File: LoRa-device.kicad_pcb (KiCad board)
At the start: 2 copper layers, 86.4 x 50.8 mm, 90 parts, among them J1 USB_C_Receptacle_USB2.0_14P, J2 Conn_01x02_Pin, J3 Conn_01x12_Pin, J4 Conn_01x14_Pin, J6 Conn_01x04_Pin, Q1 AO3401A, Q2 S8050, U1 ESP32-S3, U2 W25Q128JVS, U3 MCP73831-2-OT, U4 AMS1117-3.3, U5 Ai-Thinker-Ra-01, U6 BME280, U7 L70-R, Y1 32.768 kHz, Y2 40MHz(10ppm)

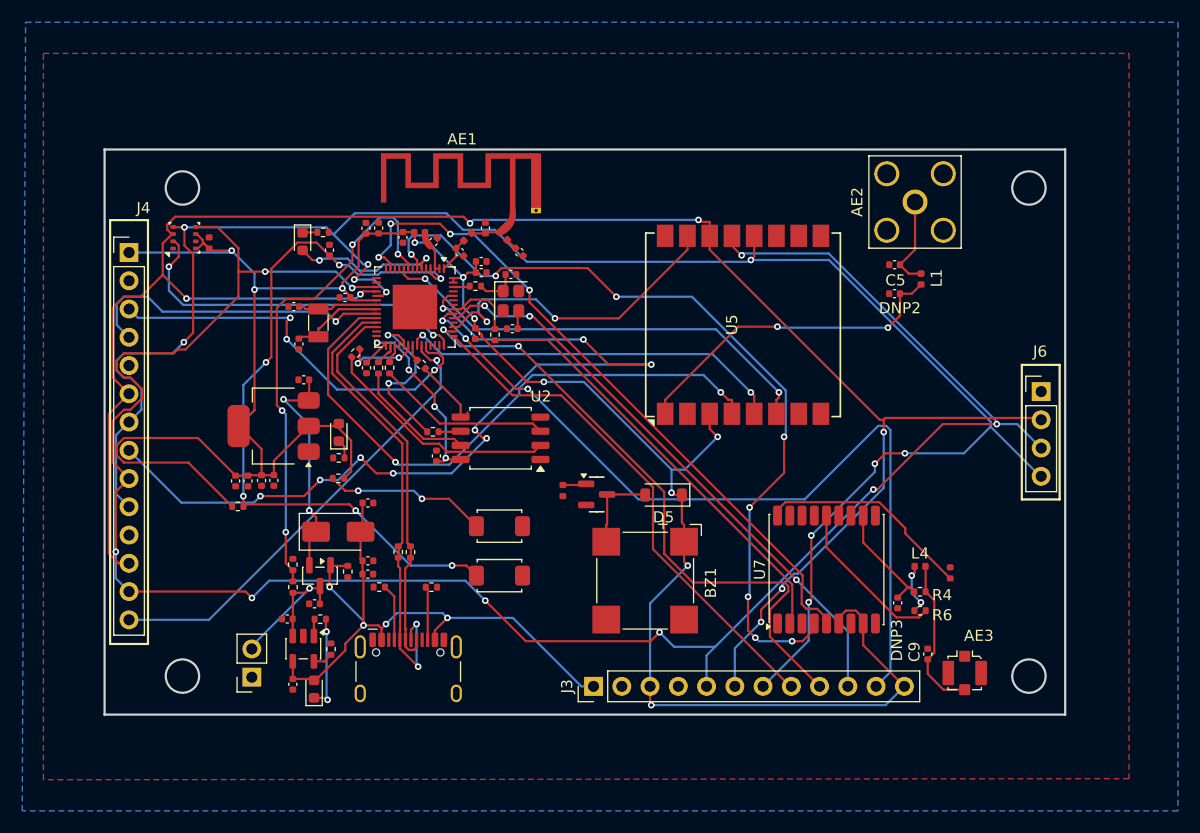
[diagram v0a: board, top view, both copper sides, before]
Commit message: First routing
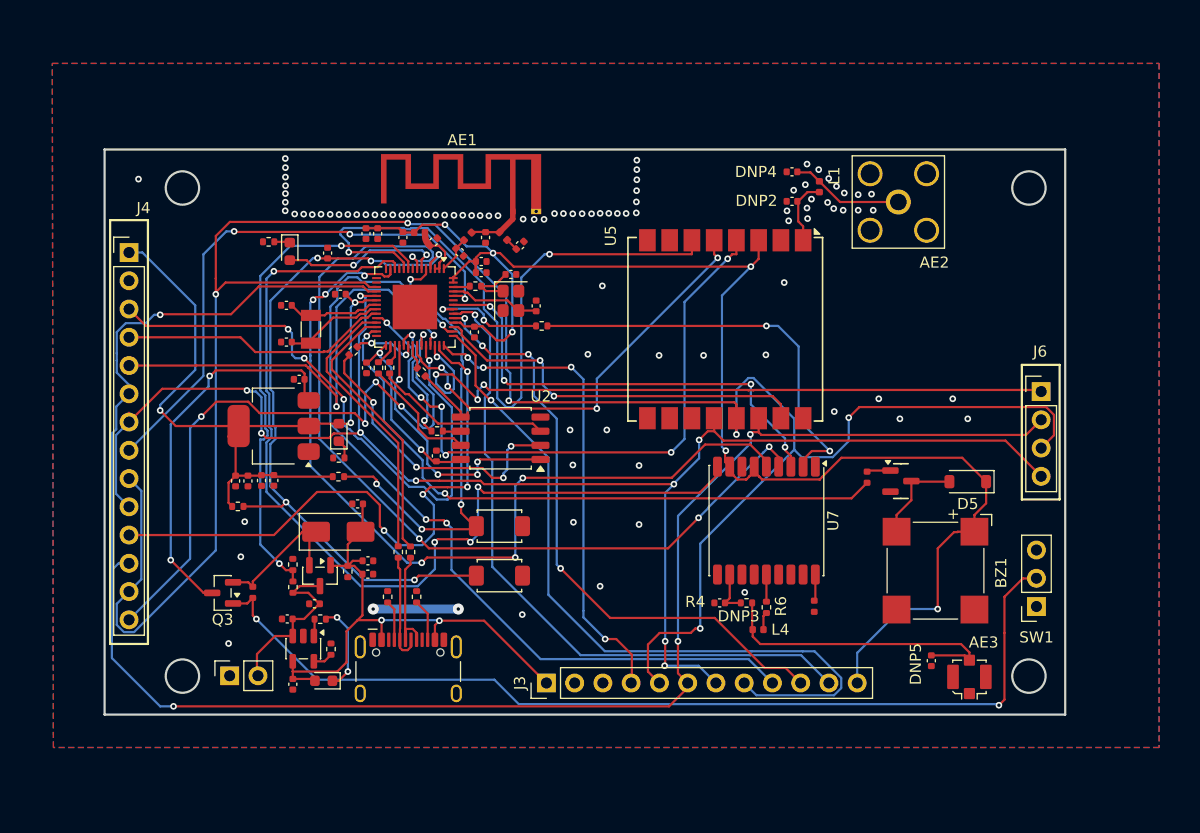
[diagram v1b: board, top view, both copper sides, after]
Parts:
- removed C1: 100nF, PCM_JLCPCB:C_0402
- removed C5, C9: 15pF, Capacitor_SMD:C_0402_1005Metric
- removed U6: BME280, PCM_JLCPCB:Bosch_LGA-8_2.5x2.5mm_P0.65mm_ClockwisePinNumbering
- added DNP4: ~, Capacitor_SMD:C_0402_1005Metric, F.Cu at (163.7, 75.8)
- added DNP5: ~, Capacitor_SMD:C_0402_1005Metric, F.Cu at (176.2, 119.8)
- added Q3: AO3401A, Package_TO_SOT_SMD:SOT-23, F.Cu at (112.5, 113.7)
- added R7: 100kΩ, PCM_JLCPCB:R_0402, F.Cu at (115.2, 113.7)
- added SW1: SW_Nidec_CAS-120A1, Connector_PinSocket_2.54mm:PinSocket_1x03_P2.54mm_Vertical, F.Cu at (185.7, 114.9)
- DNP2, DNP3: value 15pF -> ~
- moved Q2 27.4 mm to (173.5, 103.7)
- moved D5 27.4 mm to (179.5, 103.7)
- moved R5 27.4 mm to (170.4, 103.3)
- moved BZ1 26.1 mm to (176.6, 111.7)
- moved DNP3 16.0 mm to (157.2, 114.6), turned to 180 degrees
- moved L4 15.6 mm to (160.7, 117.0), turned to 180 degrees
- moved R4 15.6 mm to (159.6, 114.6)
- moved R6 13.8 mm to (161.4, 115.0), turned to 90 degrees
- moved R3 12.6 mm to (165.7, 114.9), turned to -90 degrees
- moved DNP2 12.4 mm to (163.7, 78.5)
- moved L1 12.3 mm to (166.2, 77.2)
- moved U7 6.97 mm to (161.4, 107.2), turned to -90 degrees
- moved R25 4.97 mm to (116.7, 82.1), turned to 180 degrees
- moved R24 4.27 mm to (141.2, 89.7), turned to 0 degrees
- moved J3 4.25 mm to (141.6, 121.8)
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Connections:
- C7 pad 1: VSYS -> VSYS_SW
- J3 pad 3: VDD_CPU -> GND
- J3 pad 4: GND -> IO37
- U4 pad 3: VSYS -> VSYS_SW
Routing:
- net Net-(Q3-G): track 0.00 -> 87.5 mm, vias 0 -> 2
- net IO7: track 0.00 -> 85.9 mm, vias 0 -> 4
- net IO35: track 0.00 -> 64.4 mm, vias 0 -> 4
- net IO21: track 0.00 -> 57.4 mm, vias 0 -> 2
- net IO36: track 0.00 -> 54.9 mm, vias 0 -> 4
- net IO34: track 0.00 -> 41.8 mm, vias 0 -> 2
- net RX: track 0.00 -> 41.8 mm, vias 0 -> 4
- net VSYS_SW: track 0.00 -> 34.9 mm, vias 0 -> 2
- net IO14/SCK: track 171.6 -> 141.0 mm, vias 10 -> 9
- net IO46: track 80.1 -> 50.1 mm, vias 9 -> 3
- net IO0: track 14.7 -> 41.4 mm, vias 2 -> 4
- net IO5: track 40.7 -> 65.1 mm
- net Net-(U5-ANT): track 29.8 -> 5.93 mm, vias 2 -> 0
- net SPICS0: track 0.00 -> 23.8 mm, vias 0 -> 4
- net IO39: track 56.3 -> 77.0 mm, vias 2 -> 3
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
